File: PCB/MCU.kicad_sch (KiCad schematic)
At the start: 9 parts, among them J1 UJ20-C-H-G-SMT-2A-P16-TR, J2 Conn_01x05_Pin, SW1 SKRKAHE020, U1 RAK4630, U2 USBLC6-2SC6

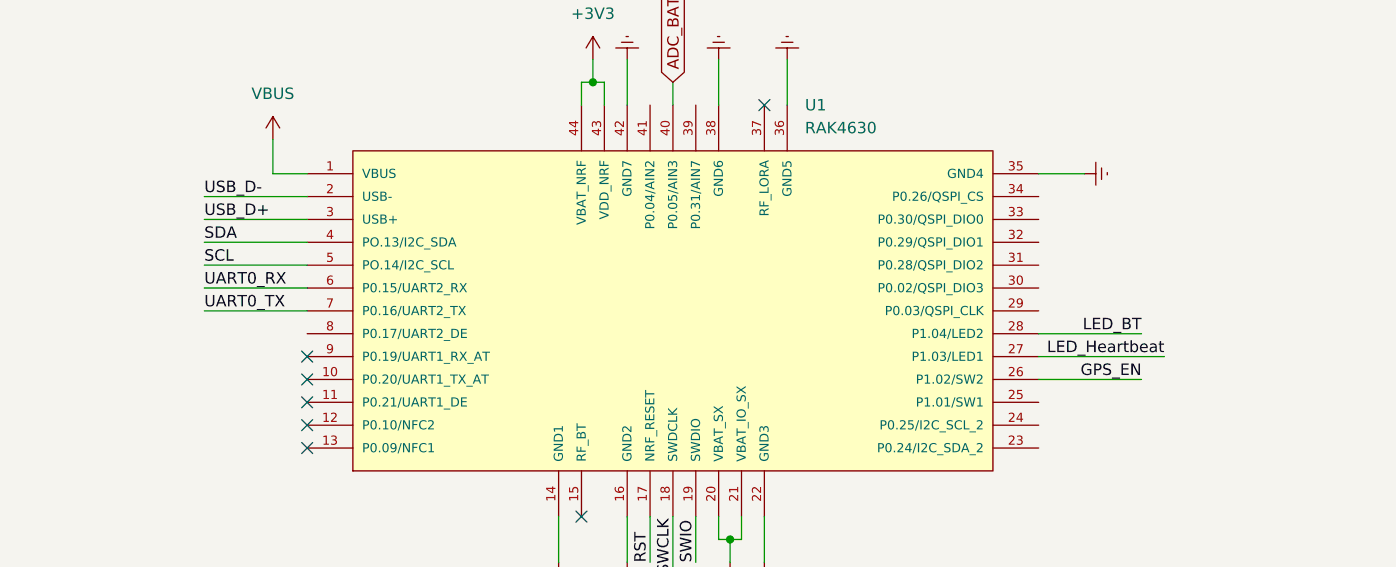
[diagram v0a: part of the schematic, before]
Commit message: a bit of work on the pheripherials
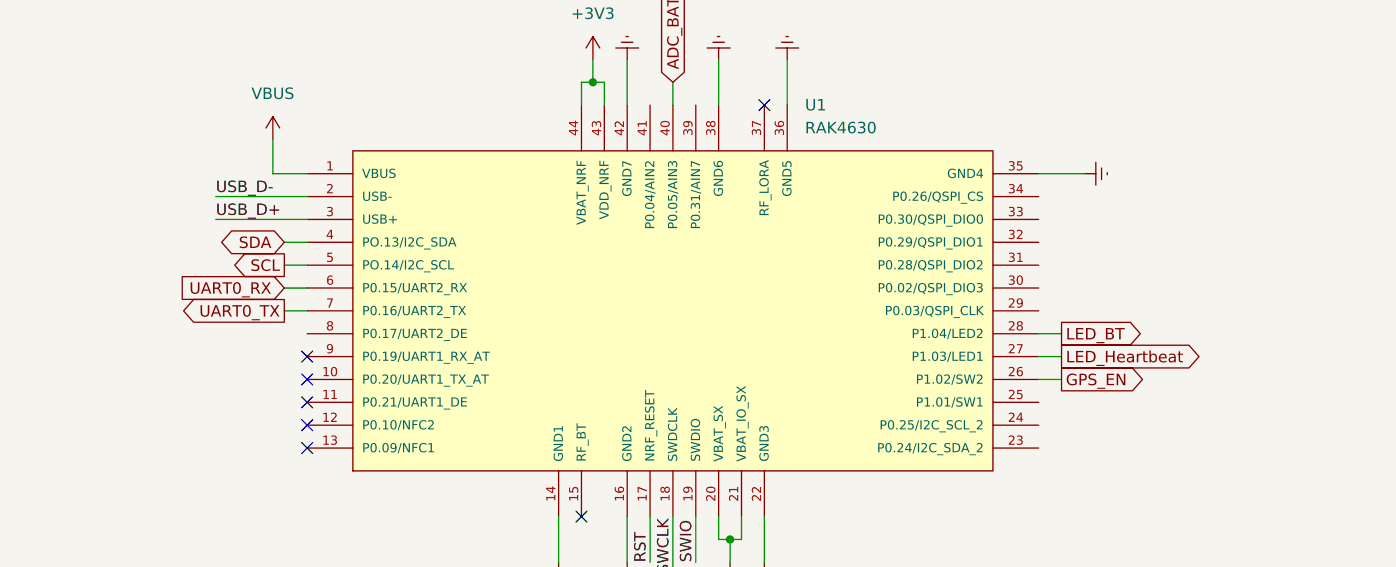
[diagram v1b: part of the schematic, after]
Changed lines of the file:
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@@
-	(wire
-		(pts
-			(xy 85.09 69.85) (xy 73.66 69.85)
-		)
-		(stroke
-			(width 0)
-			(type default)
-		)
-	)
 	(wire
 		(pts
@@
 	(wire
 		(pts
-			(xy 73.66 57.15) (xy 85.09 57.15)
+			(xy 74.93 57.15) (xy 85.09 57.15)
 		)
 		(stroke
@@
 	(wire
 		(pts
-			(xy 85.09 62.23) (xy 73.66 62.23)
+			(xy 85.09 62.23) (xy 82.55 62.23)
 		)
 		(stroke
@@
 	(wire
 		(pts
-			(xy 85.09 64.77) (xy 73.66 64.77)
+			(xy 85.09 64.77) (xy 82.55 64.77)
 		)
 		(stroke
@@
 	(wire
 		(pts
-			(xy 166.37 74.93) (xy 180.34 74.93)
-		)
-		(stroke
-			(width 0)
-			(type default)
-		)
-	)
-	(wire
-		(pts
-			(xy 166.37 77.47) (xy 177.8 77.47)
+			(xy 166.37 74.93) (xy 168.91 74.93)
+		)
+		(stroke
+			(width 0)
+			(type default)
+		)
+	)
+	(wire
+		(pts
+			(xy 166.37 77.47) (xy 168.91 77.47)
+		)
+		(stroke
+			(width 0)
+			(type default)
+		)
+	)
+	(wire
+		(pts
+			(xy 82.55 69.85) (xy 85.09 69.85)
 		)
 		(stroke
@@
 	(wire
 		(pts
-			(xy 85.09 67.31) (xy 73.66 67.31)
+			(xy 85.09 67.31) (xy 82.55 67.31)
 		)
 		(stroke
@@
 	(wire
 		(pts
-			(xy 166.37 72.39) (xy 177.8 72.39)
+			(xy 166.37 72.39) (xy 168.91 72.39)
 		)
 		(stroke
@@
 	(wire
 		(pts
-			(xy 73.66 59.69) (xy 85.09 59.69)
+			(xy 74.93 59.69) (xy 85.09 59.69)
 		)
 		(stroke
@@
 		)
 	)
-	(label "USB_D-"
-		(at 73.66 57.15 0)
-		(effects
-			(font
-				(size 1.27 1.27)
-			)
-			(justify left bottom)
-		)
-	)
 	(label "SCL"
 		(at 236.22 36.83 0)
@@
 		)
 	)
+	(label "USB_D+"
+		(at 74.93 59.69 0)
+		(effects
+			(font
+				(size 1.27 1.27)
+			)
+			(justify left bottom)
+		)
+	)
 	(label "UART0_RX"
 		(at 236.22 21.59 0)
@@
 		)
 	)
-	(label "UART0_TX"
-		(at 73.66 69.85 0)
-		(effects
-			(font
-				(size 1.27 1.27)
-			)
-			(justify left bottom)
-		)
-	)
 	(label "D-"
 		(at 48.26 160.02 0)
@@
 		)
 	)
-	(label "LED_BT"
-		(at 177.8 72.39 180)
-		(effects
-			(font
-				(size 1.27 1.27)
-			)
-			(justify right bottom)
-		)
-	)
 	(label "GNDREF"
 		(at 240.03 149.86 180)
@@
 		)
 	)
-	(label "USB_D+"
-		(at 73.66 59.69 0)
-		(effects
-			(font
-				(size 1.27 1.27)
-			)
-			(justify left bottom)
-		)
-	)
-	(label "UART0_RX"
-		(at 73.66 67.31 0)
-		(effects
-			(font
-				(size 1.27 1.27)
-			)
-			(justify left bottom)
-		)
-	)
 	(label "SWCLK"
 		(at 125.73 99.06 90)
@@
 		)
 	)
-	(label "SCL"
-		(at 73.66 64.77 0)
-		(effects
-			(font
-				(size 1.27 1.27)
-			)
-			(justify left bottom)
-		)
-	)
-	(label "GPS_EN"
-		(at 177.8 77.47 180)
-		(effects
-			(font
-				(size 1.27 1.27)
-			)
-			(justify right bottom)
-		)
-	)
 	(label "RST"
 		(at 251.46 135.89 0)
@@
 		)
 	)
-	(label "SDA"
-		(at 73.66 62.23 0)
-		(effects
-			(font
-				(size 1.27 1.27)
-			)
-			(justify left bottom)
-		)
-	)
 	(label "RST"
 		(at 123.19 97.79 90)
@@
 		)
 	)
-	(label "LED_Heartbeat"
-		(at 180.34 74.93 180)
-		(effects
-			(font
-				(size 1.27 1.27)
-			)
-			(justify right bottom)
+	(label "USB_D-"
+		(at 74.93 57.15 0)
+		(effects
+			(font
+				(size 1.27 1.27)
+			)
+			(justify left bottom)
 		)
 	)
@@
 			)
 			(justify right bottom)
+		)
+	)
+	(global_label "SCL"
+		(shape output)
+		(at 82.55 64.77 180)
+		(fields_autoplaced yes)
+		(effects
+			(font
+				(size 1.27 1.27)
+			)
+			(justify right)
+		)
+		(property "Intersheetrefs" "${INTERSHEET_REFS}"
+			(at 76.0572 64.77 0)
+			(hide yes)
+			(show_name no)
+			(do_not_autoplace no)
+			(effects
+				(font
+					(size 1.27 1.27)
+				)
+				(justify right)
+			)
+		)
+	)
+	(global_label "LED_BT"
+		(shape output)
+		(at 168.91 72.39 0)
+		(fields_autoplaced yes)
+		(effects
+			(font
+				(size 1.27 1.27)
+			)
+			(justify left)
+		)
+		(property "Intersheetrefs" "${INTERSHEET_REFS}"
+			(at 178.5475 72.39 0)
+			(hide yes)
+			(show_name no)
+			(do_not_autoplace no)
+			(effects
+				(font
+					(size 1.27 1.27)
+				)
+				(justify left)
+			)
+		)
+	)
+	(global_label "LED_Heartbeat"
+		(shape output)
+		(at 168.91 74.93 0)
+		(fields_autoplaced yes)
+		(effects
+			(font
+				(size 1.27 1.27)
+			)
+			(justify left)
+		)
+		(property "Intersheetrefs" "${INTERSHEET_REFS}"
+			(at 185.5022 74.93 0)
+			(hide yes)
+			(show_name no)
+			(do_not_autoplace no)
+			(effects
+				(font
+					(size 1.27 1.27)
+				)
+				(justify left)
+			)
+		)
+	)
+	(global_label "UART0_RX"
+		(shape input)
+		(at 82.55 67.31 180)
+		(fields_autoplaced yes)
+		(effects
+			(font
+				(size 1.27 1.27)
+			)
+			(justify right)
+		)
+		(property "Intersheetrefs" "${INTERSHEET_REFS}"
+			(at 70.2515 67.31 0)
+			(hide yes)
+			(show_name no)
+			(do_not_autoplace no)
+			(effects
+				(font
+					(size 1.27 1.27)
+				)
+				(justify right)
+			)
+		)
+	)
+	(global_label "GPS_EN"
+		(shape output)
+		(at 168.91 77.47 0)
+		(fields_autoplaced yes)
+		(effects
+			(font
+				(size 1.27 1.27)
+			)
+			(justify left)
+		)
+		(property "Intersheetrefs" "${INTERSHEET_REFS}"
+			(at 179.0918 77.47 0)
+			(hide yes)
+			(show_name no)
+			(do_not_autoplace no)
+			(effects
+				(font
+					(size 1.27 1.27)
+				)
+				(justify left)
+			)
+		)
+	)
+	(global_label "UART0_TX"
+		(shape output)
+		(at 82.55 69.85 180)
+		(fields_autoplaced yes)
+		(effects
+			(font
+				(size 1.27 1.27)
+			)
+			(justify right)
+		)
+		(property "Intersheetrefs" "${INTERSHEET_REFS}"
+			(at 70.5539 69.85 0)
+			(hide yes)
+			(show_name no)
+			(do_not_autoplace no)
+			(effects
+				(font
+					(size 1.27 1.27)
+				)
+				(justify right)
+			)
 		)
 	)
@@
 			)
 		)
+	)
+	(global_label "SDA"
+		(shape bidirectional)
+		(at 82.55 62.23 180)
+		(fields_autoplaced yes)
+		(effects
+			(font
+				(size 1.27 1.27)
+			)
+			(justify right)
+		)
+		(property "Intersheetrefs" "${INTERSHEET_REFS}"
+			(at 74.8854 62.23 0)
+			(hide yes)
+			(show_name no)
+			(do_not_autoplace no)
+			(effects
+				(font
+					(size 1.27 1.27)
+				)
+				(justify right)
+			)
+		)
